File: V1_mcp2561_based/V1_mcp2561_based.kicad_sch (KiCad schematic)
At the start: 19 parts, among them J2 Screw_Terminal_01x02, U4 ESP32-S3-DevKitC

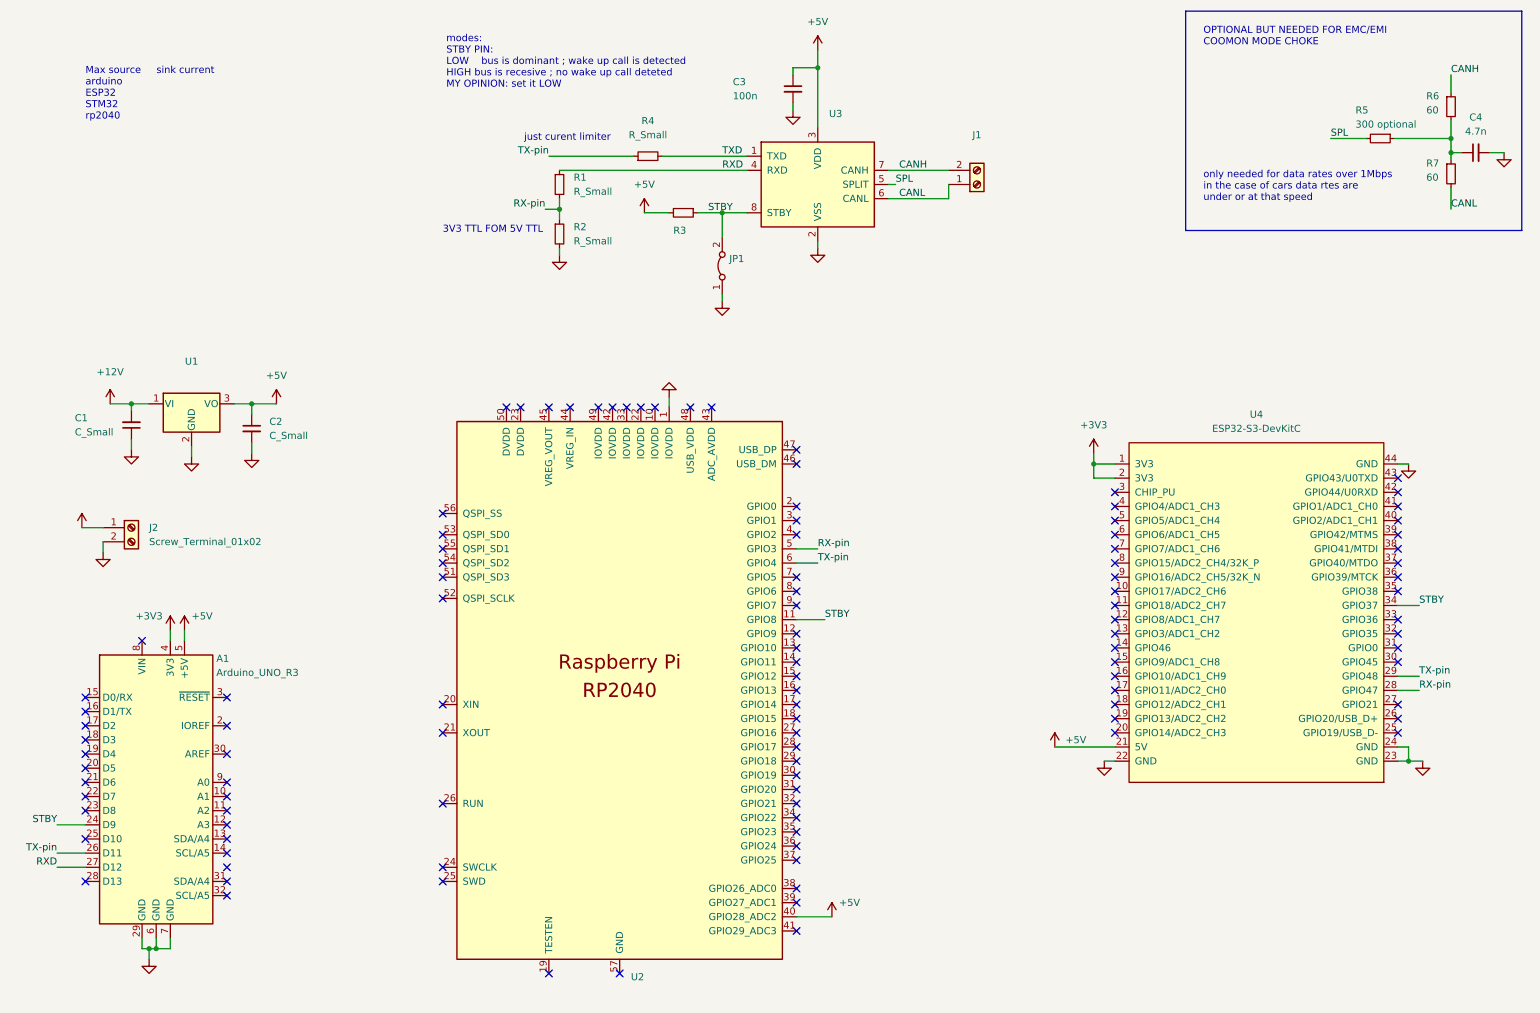
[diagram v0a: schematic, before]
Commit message: h
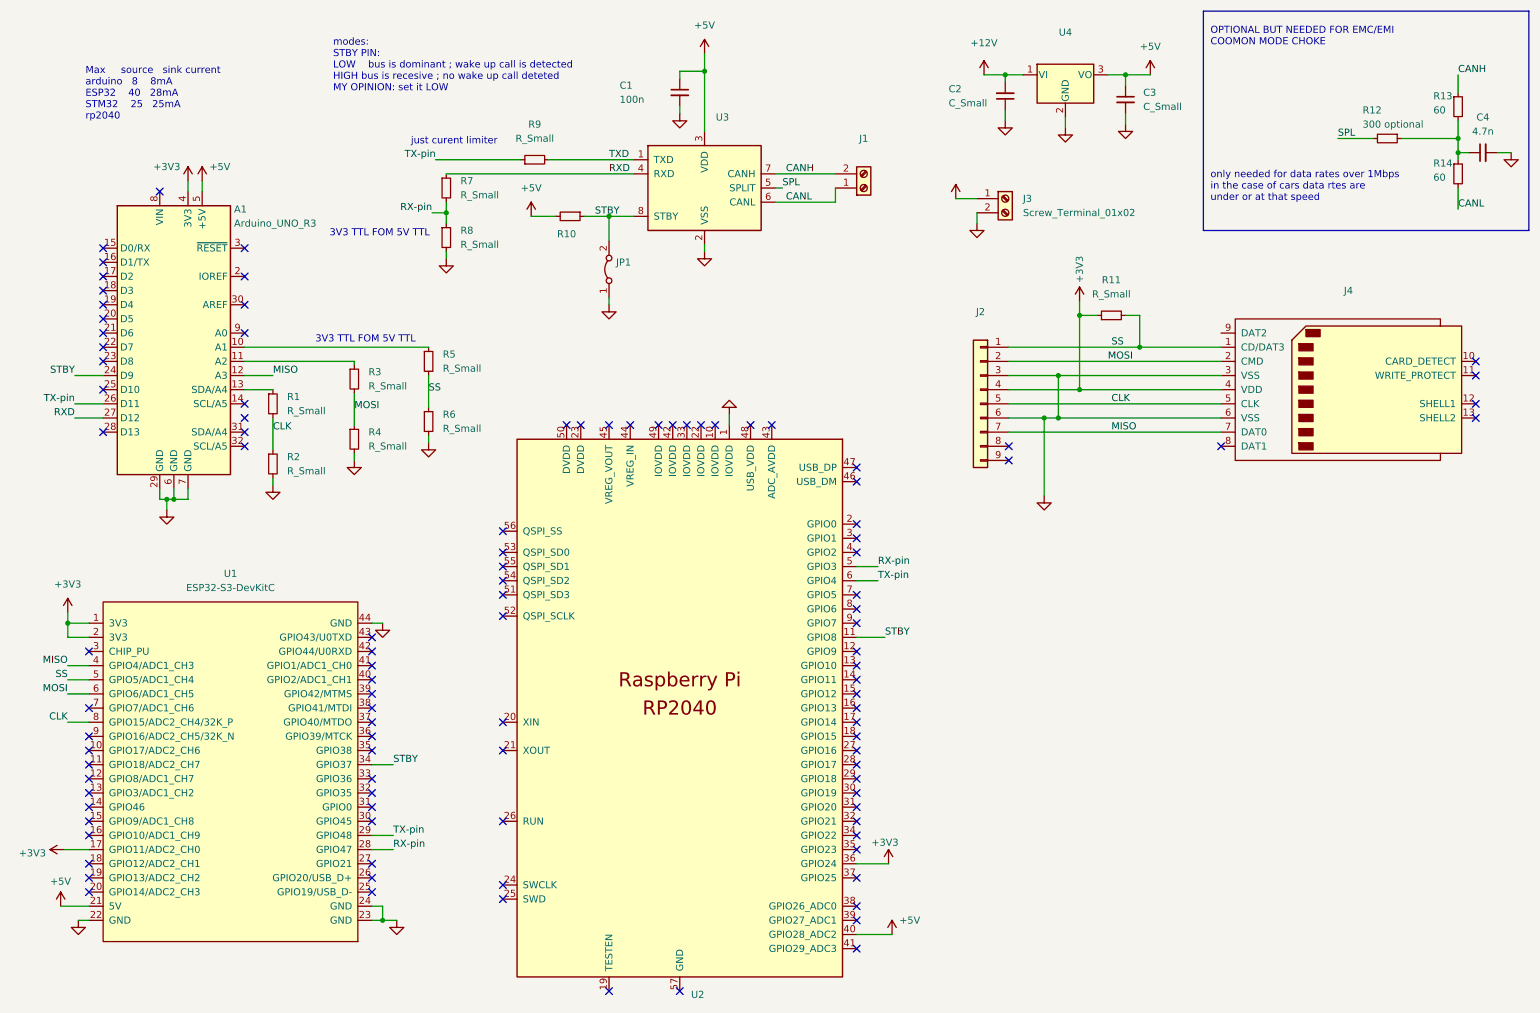
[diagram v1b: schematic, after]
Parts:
- added J2: (no value), symbol Connector_Generic:Conn_01x09
- added J4: (no value), symbol Connector:SD_Card
- added R1, R11, R2, R3, R4, R5, R6: R_Small, Resistor_THT:R_Axial_DIN0204_L3.6mm_D1.6mm_P5.08mm_Horizontal, symbol Device:R_Small
- renumbered C3 to C1, C1 to C2, C2 to C3, J2 to J3, R3 to R10, R5 to R12, R6 to R13, R7 to R14, R1 to R7, R2 to R8, R4 to R9, U4 to U1, U1 to U4
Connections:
- net +3V3: now also U1.17 (GPIO11/ADC2_CH0), U2.36 (GPIO24), J2.4 (Pin_4), J4.4 (VDD), R11.1
- net GND: now also J2.3 (Pin_3), J2.6 (Pin_6), J4.3 (VSS), J4.6 (VSS), R2.2, R4.2, R6.2
- net at A1.10 (A1): now also R5.1
- net at A1.11 (A2): now also R3.1
- net MISO: now reaches A1.12 (A3)
- net MISO: now also U1.4 (GPIO4/ADC1_CH3), J2.7 (Pin_7), J4.7 (DAT0)
- net at A1.13 (SDA/A4): now also R1.1
- net SS: now reaches U1.5 (GPIO5/ADC1_CH4)
- net SS: now also J2.1 (Pin_1), J4.1 (CD/DAT3), R11.2, R5.2, R6.1
- net MOSI: now reaches U1.6 (GPIO6/ADC1_CH5)
- net MOSI: now also J2.2 (Pin_2), J4.2 (CMD), R3.2, R4.1
- net CLK: now reaches U1.8 (GPIO15/ADC2_CH4/32K_P)
- net CLK: now also J2.5 (Pin_5), J4.5 (CLK), R1.2, R2.1
- no-connect marks 110 -> 107
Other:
- note added: "Max source sink current arduino 8 8mA ESP32 40 28mA STM32 25 25mA rp2040"
- note removed: "Max source sink current arduino ESP32 STM32 rp2040"
- moved on the sheet: A1, C1, C2, C3, C4, J1, J3, JP1, R10, R12, R13, R14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
